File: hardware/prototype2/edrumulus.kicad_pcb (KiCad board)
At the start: 2 copper layers, 83 parts, among them J1 Snare, J10 DIN-5, J11 DIN-5, J2 Hi-Hat, J3 Crash, J4 Ride, J5 Kick, J6 Tom1, J7 Tom2, J8 Tom3, J9 Hi-Hat Ctrl, U1 ESP32-DEVKIT-V1, U2 6N138

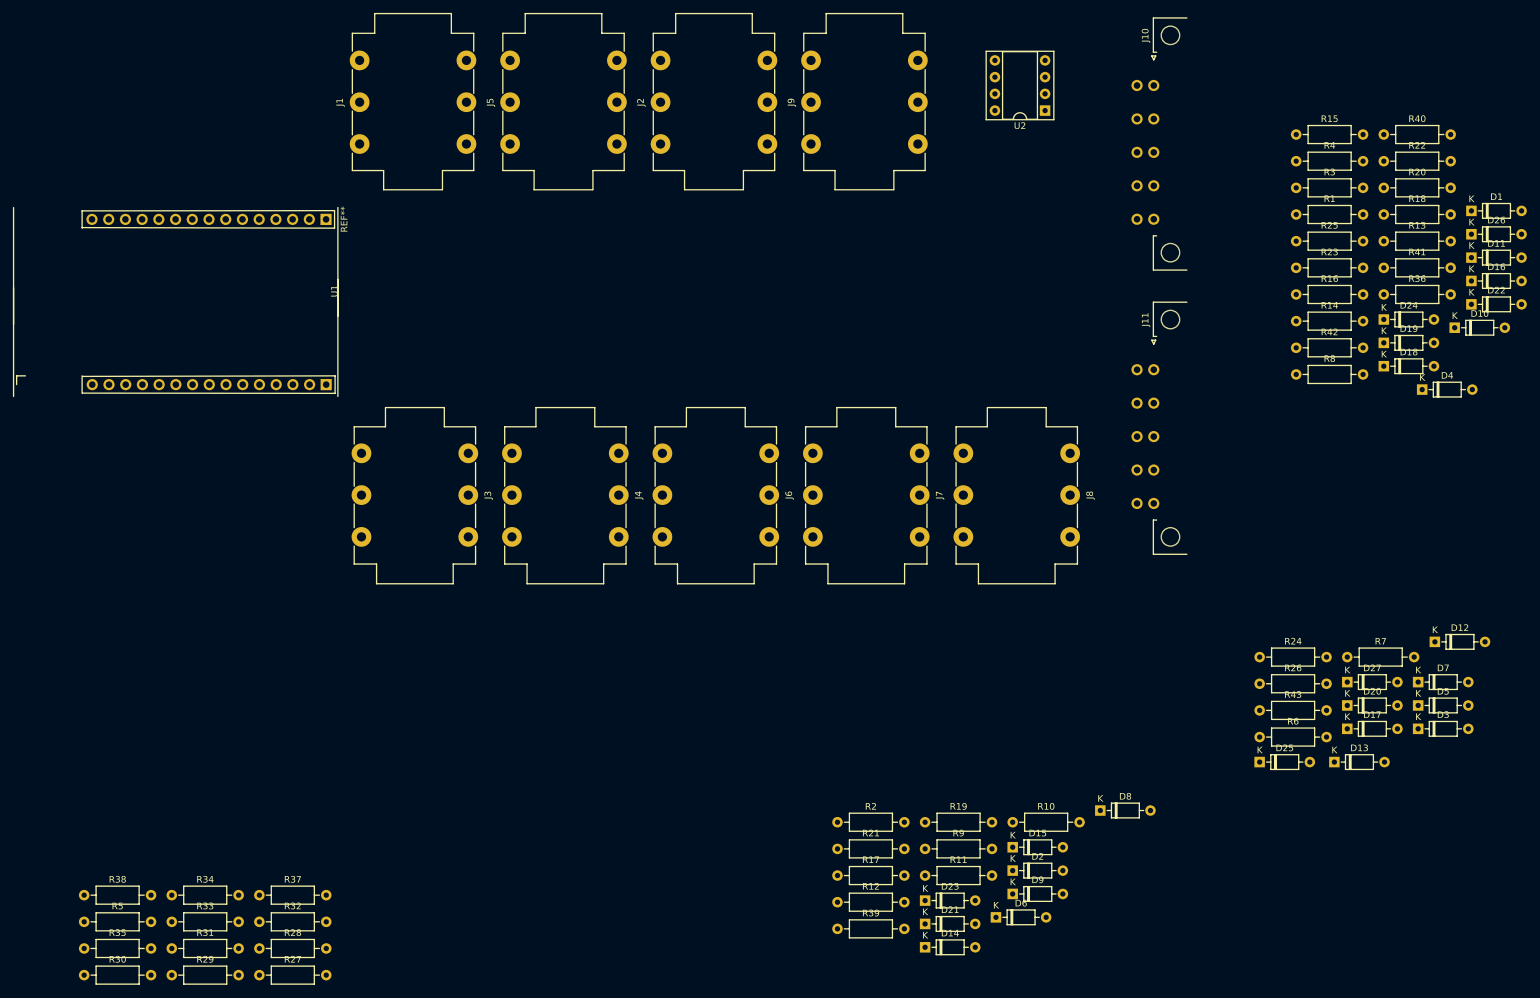
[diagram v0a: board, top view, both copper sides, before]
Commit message: some tests, moving components
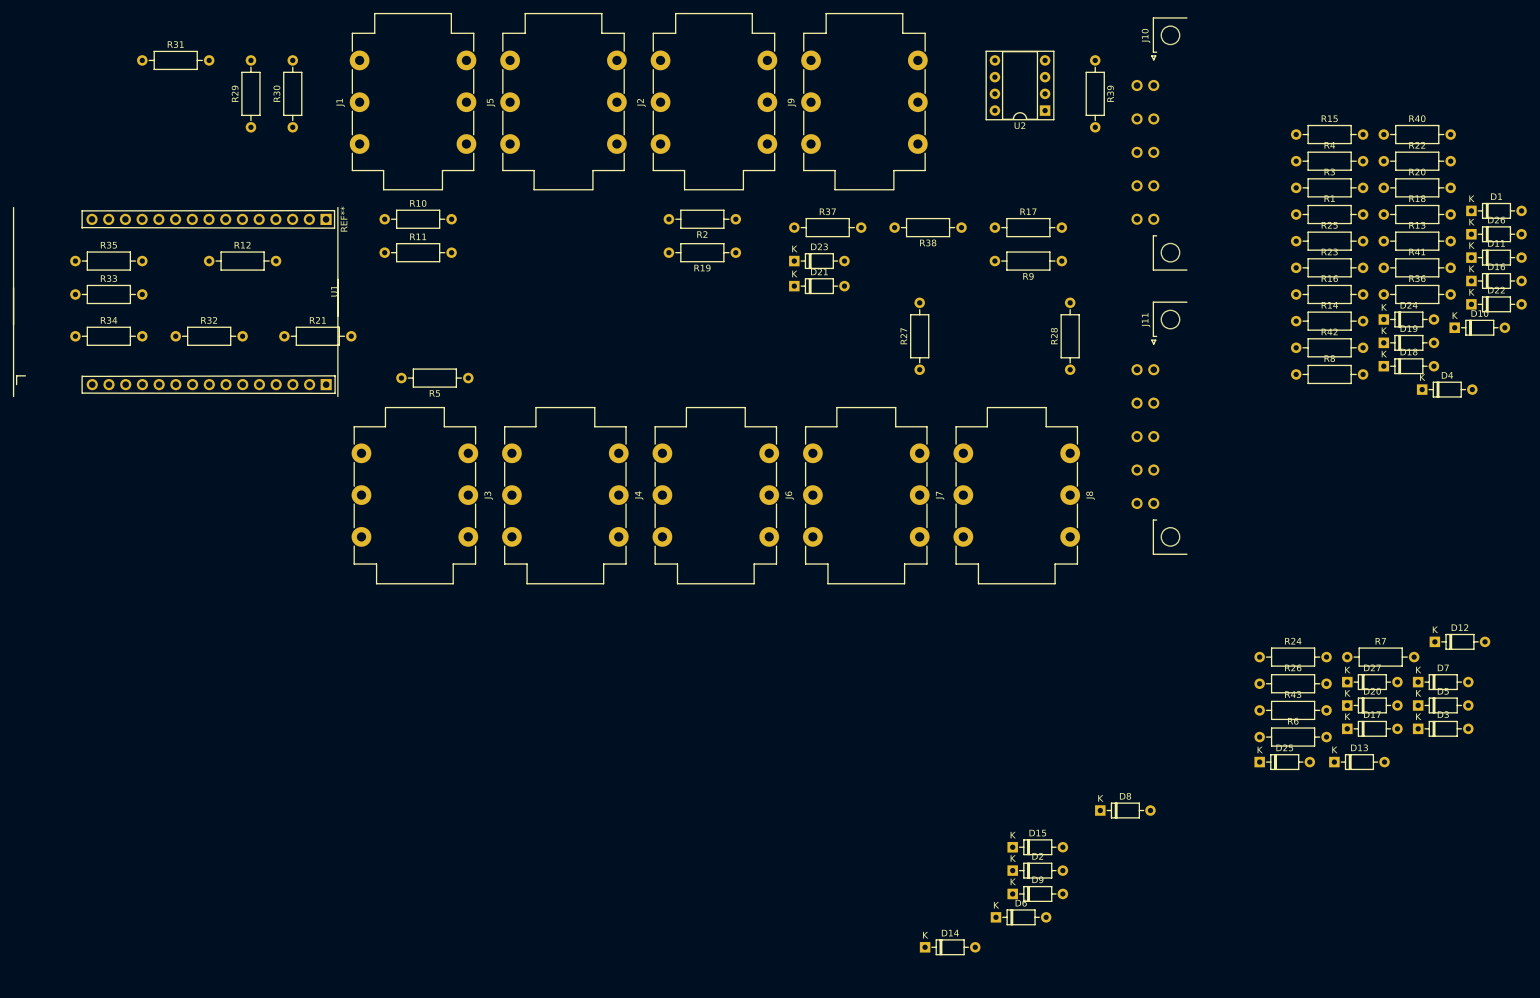
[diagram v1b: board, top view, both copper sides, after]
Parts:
- moved R38 167.5 mm to (179.1, 55.9), turned to 180 degrees
- moved R28 151.3 mm to (195.6, 77.5), turned to 90 degrees
- moved R39 137.6 mm to (199.4, 30.5), turned to 270 degrees
- moved R12 136.4 mm to (64.8, 61.0)
- moved R27 136.1 mm to (172.7, 77.5), turned to 90 degrees
- moved R31 135.0 mm to (54.6, 30.5)
- moved R30 132.7 mm to (77.5, 40.6), turned to 90 degrees
- moved R10 132.3 mm to (91.4, 54.6)
- moved R37 130.0 mm to (153.7, 55.9)
- moved R29 129.4 mm to (71.1, 40.6), turned to 90 degrees
- moved R11 125.3 mm to (91.4, 59.7)
- moved R21 114.6 mm to (76.2, 72.4)
- moved R35 104.4 mm to (44.5, 61.0)
- moved R17 101.3 mm to (184.2, 55.9)
- moved R5 101.1 mm to (104.1, 78.7), turned to 180 degrees
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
